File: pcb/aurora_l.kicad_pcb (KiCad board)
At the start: 2 copper layers, 123.1 x 132.9 mm, 96 parts

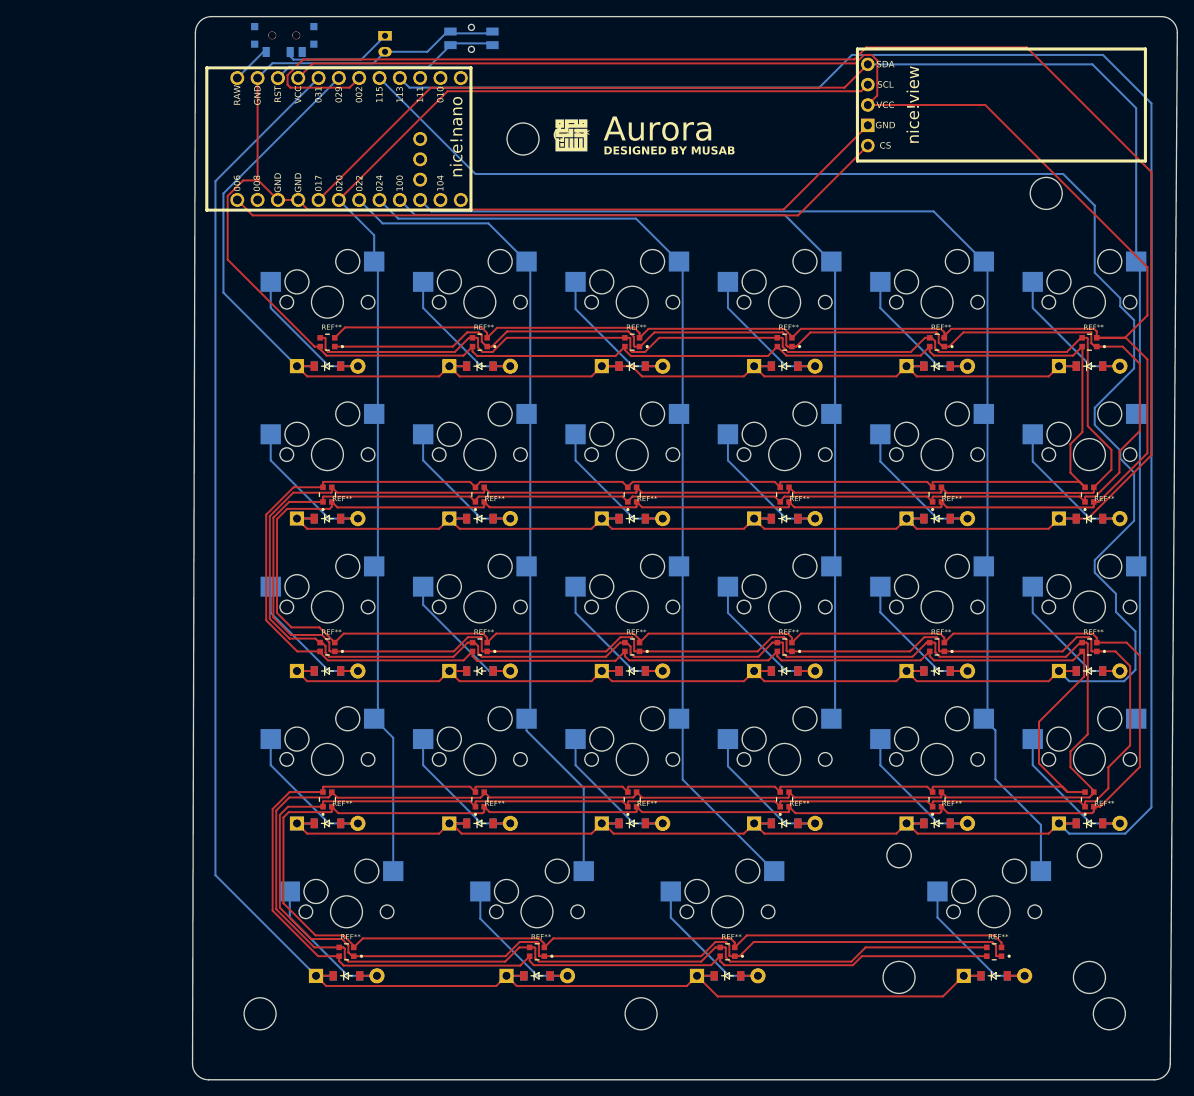
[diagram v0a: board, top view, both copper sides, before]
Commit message: Left PCB pin layout fixes and full routed pcb
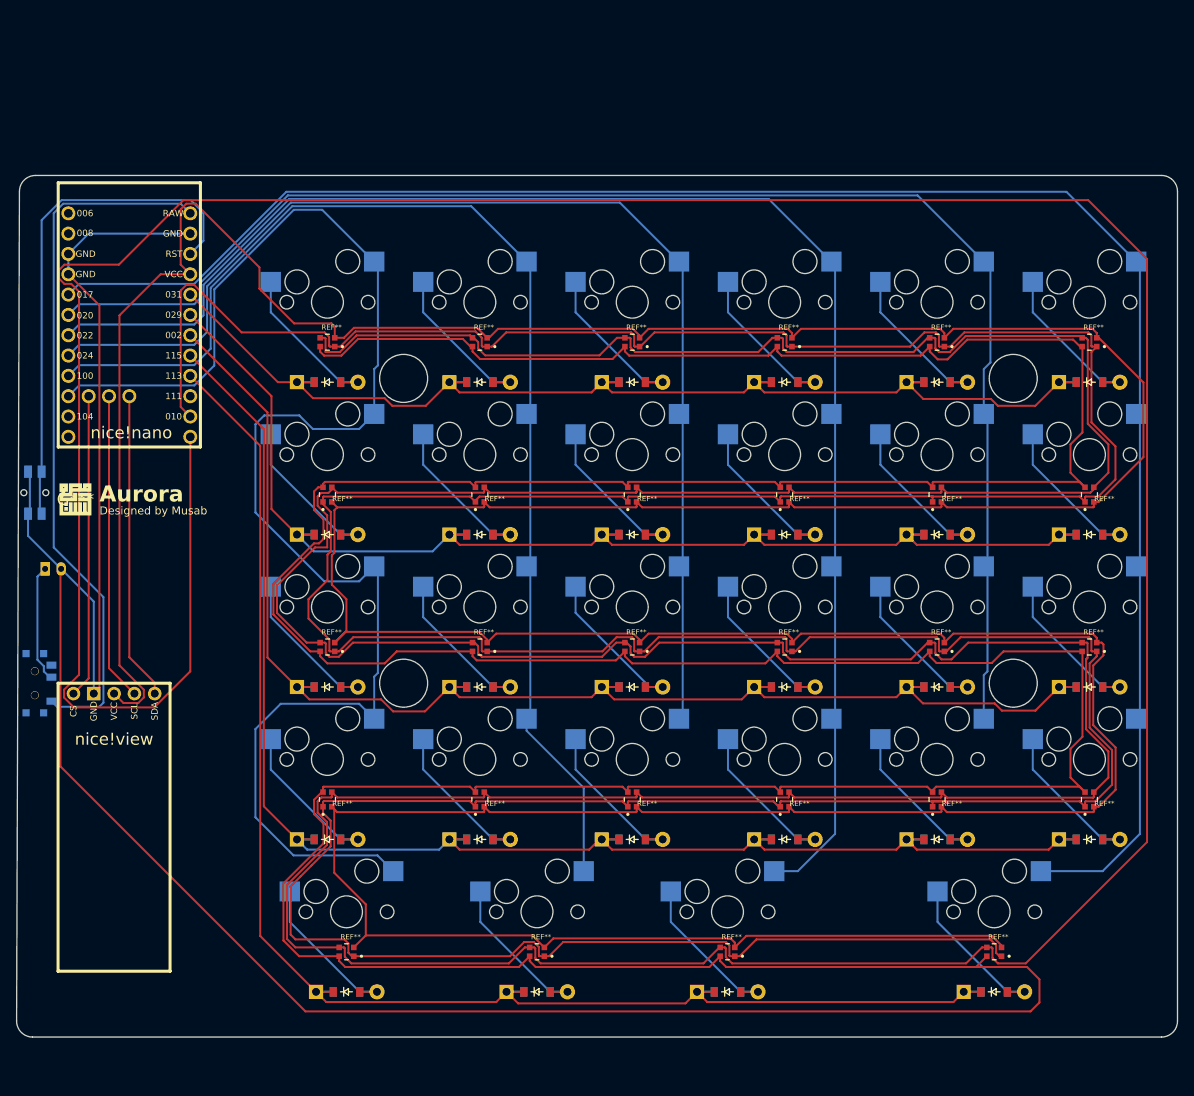
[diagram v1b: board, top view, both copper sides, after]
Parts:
- removed the ? at (139.2, 131.8)
- removed the ? at (91.6, 131.8)
- removed the ? at (124.5, 22.4)
- removed the ? at (197.7, 131.8)
- removed the ? at (189.8, 29.2)
- removed the REF** at (185.9, 113.9)
- added ?: , HOLE_M2_TH, F.Cu at (185.7, 52.4)
- added ?: , HOLE_M2_TH, F.Cu at (109.5, 90.5)
- added ?: , HOLE_M2_TH, F.Cu at (109.5, 52.4)
- added ?: , HOLE_M2_TH, F.Cu at (185.7, 90.5)
- moved niceView1 117.7 mm to (73.3, 90.5), turned to -90 degrees
- moved T1 86.8 mm to (63.4, 90.5), turned to 90 degrees
- moved B1 78.8 mm to (63.4, 66.7), turned to 90 degrees
- moved JST1 77.7 mm to (65.7, 76.2), turned to 0 degrees
- moved G*** 76.9 mm to (68.5, 67.5)
- moved MCU1 36.0 mm to (75.2, 45.7), turned to -90 degrees
- moved D25 2.00 mm to (102.4, 129.1)
- moved D26 2.00 mm to (126.2, 129.1)
- moved D27 2.00 mm to (150.0, 129.1)
- moved D28 2.00 mm to (183.3, 129.1)
- moved D1 2.00 mm to (100.0, 110.0)
- moved D10 2.00 mm to (138.1, 91.0)
- moved D11 2.00 mm to (138.1, 71.9)
- moved D12 2.00 mm to (138.1, 52.9)
- moved D13 2.00 mm to (157.2, 110.0)
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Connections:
- D1 pad 1: P113 -> P115
- D10 pad 1: P115 -> P002
- D11 pad 1: P002 -> P029
- D12 pad 1: P029 -> P031
- D13 pad 1: P113 -> P115
- D14 pad 1: P115 -> P002
- D15 pad 1: P002 -> P029
- D16 pad 1: P029 -> P031
- D17 pad 1: P113 -> P115
- D18 pad 1: P115 -> P002
- D19 pad 1: P002 -> P029
- D2 pad 1: P115 -> P002
- D20 pad 1: P029 -> P031
- D21 pad 1: P113 -> P115
- D22 pad 1: P115 -> P002
- D23 pad 1: P002 -> P029
- D24 pad 1: P029 -> P031
- D25 pad 1: P031 -> P113
- D26 pad 1: P031 -> P113
- D27 pad 1: P031 -> P113
- D28 pad 1: P031 -> P113
- D3 pad 1: P002 -> P029
- D4 pad 1: P029 -> P031
- D5 pad 1: P113 -> P115
- D6 pad 1: P115 -> P002
- D7 pad 1: P002 -> P029
- D8 pad 1: P029 -> P031
- D9 pad 1: P113 -> P115
- REF** pad 1: P8 -> P010 (x28)
- REF** pad 3: P15 -> P009 (x28)
- S1 pad 2: P020 -> P011
- S13 pad 2: P100 -> P022
- S14 pad 2: P100 -> P022
- S15 pad 2: P100 -> P022
- S16 pad 2: P100 -> P022
- S17 pad 2: P011 -> P020
- S18 pad 2: P011 -> P020
- S19 pad 2: P011 -> P020
- S2 pad 2: P020 -> P011
- S20 pad 2: P011 -> P020
- S25 pad 2: P020 -> P011
- S26 pad 2: P022 -> P100
- S27 pad 2: P024 -> P022
- S28 pad 2: P011 -> P017
- S3 pad 2: P020 -> P011
- S4 pad 2: P020 -> P011
- S5 pad 2: P022 -> P100
- S6 pad 2: P022 -> P100
- S7 pad 2: P022 -> P100
- S8 pad 2: P022 -> P100
- niceView1 pad 1: P006 -> P101
- niceView1 pad 4: P020 -> P102
- niceView1 pad 5: P017 -> P107
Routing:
- net P009: track 0.00 -> 946.9 mm
- net P010: track 0.00 -> 637.9 mm
- net P8: track 611.2 -> 0.00 mm
- net P15: track 601.1 -> 0.00 mm
- net P113: track 326.6 -> 185.1 mm
- net P002: track 301.2 -> 179.0 mm
- net GND: track 743.0 -> 862.9 mm
- net P115: track 301.5 -> 192.5 mm
- net P022: track 104.4 -> 190.3 mm
- net RAW: track 4.97 -> 88.8 mm
- net P006: track 83.2 -> 0.00 mm
- net P031: track 225.3 -> 147.1 mm
- net VCC: track 739.3 -> 675.9 mm
- net P017: track 189.0 -> 229.6 mm
- net P102: track 0.00 -> 38.5 mm
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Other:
- board size 123.1 x 132.9 mm -> 145.1 x 107.7 mm
- board text added: "Designed by Musab"
- board text removed: "DESIGNED BY MUSAB"
